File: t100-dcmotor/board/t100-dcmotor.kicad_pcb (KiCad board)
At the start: 2 copper layers, 34.5 x 99.5 mm, 24 parts, among them J1 T100-IN, J2 T100-OUT, J3 Conn_01x08_Female, U1 ATSAMD11D14A-SS, U2 TB67H451FNG, X1 SWD

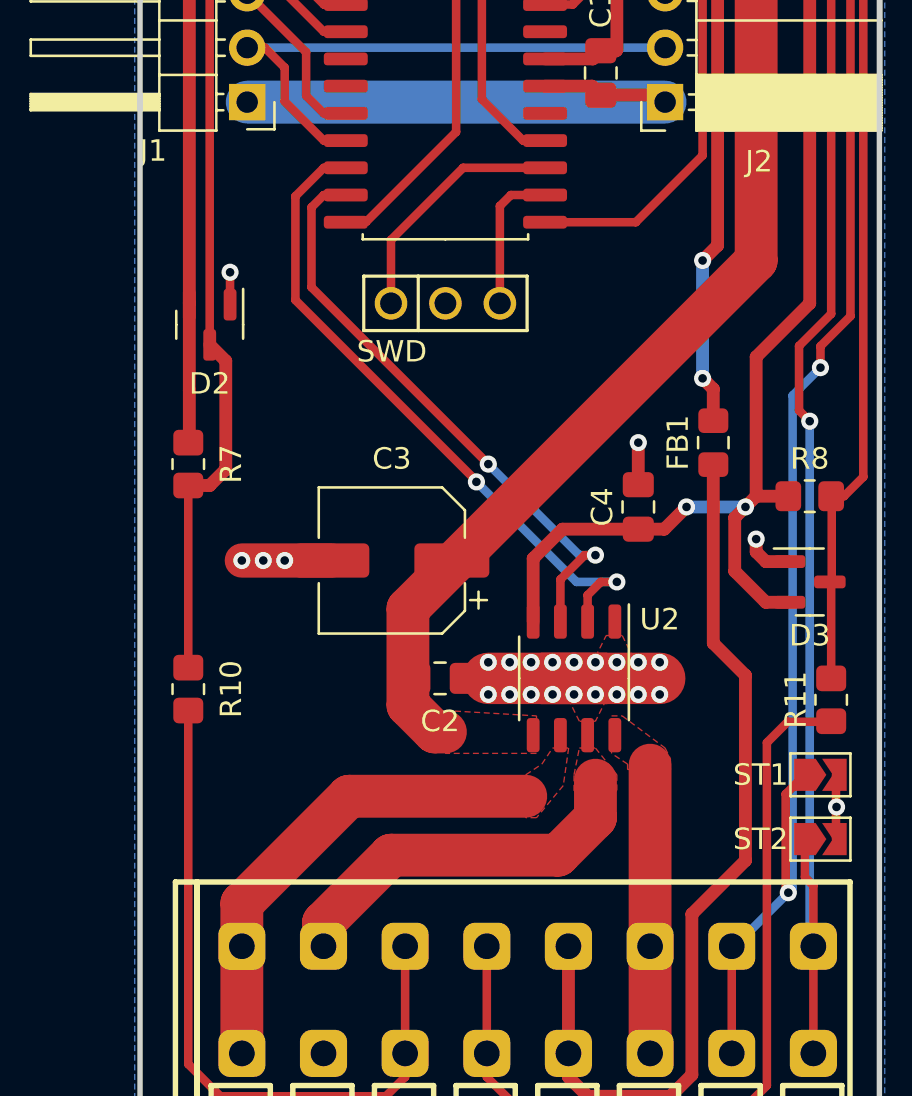
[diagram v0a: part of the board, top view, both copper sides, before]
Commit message: WIP
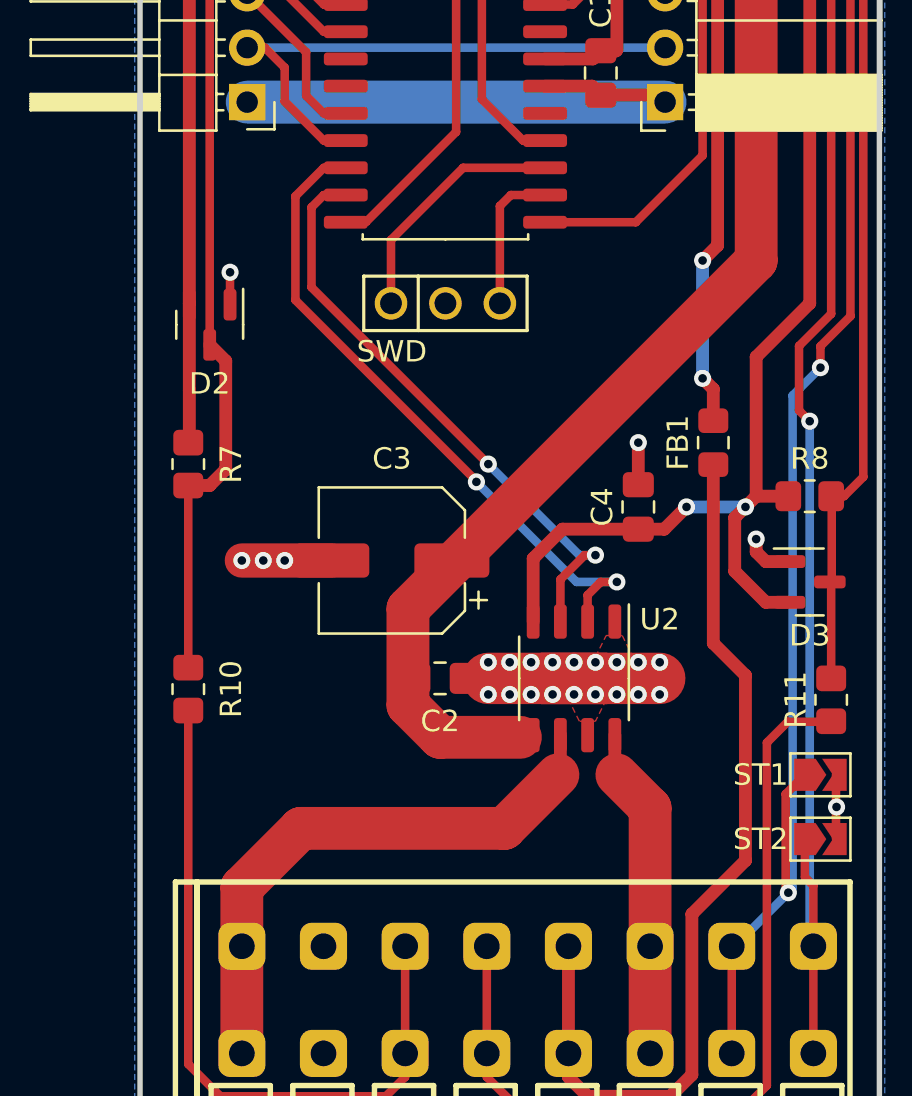
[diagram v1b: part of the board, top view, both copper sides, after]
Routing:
- net GND: track 96.9 -> 79.3 mm
- net /MOTOR_M: track 22.3 -> 26.6 mm
- net +12V: track 102.0 -> 105.6 mm
- net /MOTOR_P: track 13.5 -> 15.5 mm
- removed copper zone on F.Cu, net +12V
- removed copper zone on F.Cu, net /MOTOR_M
- removed copper zone on F.Cu, net /MOTOR_P
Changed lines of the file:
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@@
   )
   (setup
+    (stackup
+      (layer "F.SilkS" (type "Top Silk Screen") (color "White"))
+      (layer "F.Paste" (type "Top Solder Paste"))
+      (layer "F.Mask" (type "Top Solder Mask") (color "Black") (thickness 0.01))
+      (layer "F.Cu" (type "copper") (thickness 0.035))
+      (layer "dielectric 1" (type "core") (thickness 1.51) (material "FR4") (epsilon_r 4.5) (loss_tangent 0.02))
+      (layer "B.Cu" (type "copper") (thickness 0.035))
+      (layer "B.Mask" (type "Bottom Solder Mask") (color "Black") (thickness 0.01))
+      (layer "B.Paste" (type "Bottom Solder Paste"))
+      (layer "B.SilkS" (type "Bottom Silk Screen") (color "White"))
+      (copper_finish "None")
+      (dielectric_constraints no)
+    )
     (pad_to_mask_clearance 0.051)
     (solder_mask_min_width 0.25)
@@
     (property "Sheetname" "")
     (attr through_hole)
-    (fp_text reference "J1" (at 4.385 -2.27 180) (layer "F.SilkS")
+    (fp_text reference "J1" (at 4.385 -2.27 180) (layer "F.SilkS") hide
       (effects (font (size 1 1) (thickness 0.15)))
     )
@@
     (property "Sheetname" "")
     (attr through_hole)
-    (fp_text reference "J2" (at -4.38 -2.77 180) (layer "F.SilkS")
+    (fp_text reference "J2" (at -4.38 -2.77 180) (layer "F.SilkS") hide
       (effects (font (size 1 1) (thickness 0.15)))
     )
@@
   (segment (start 106.915 84.775) (end 107.25 85.11) (width 0.6) (layer "F.Cu") (net 1))
   (segment (start 113 106.55) (end 111.95 106.55) (width 0.6) (layer "F.Cu") (net 1))
-  (segment (start 91.31 124.5) (end 91.31 123.4) (width 2) (layer "F.Cu") (net 1))
   (segment (start 103 112) (end 107 112) (width 2.4) (layer "F.Cu") (net 1))
   (segment (start 115.225 117.975) (end 115.225 119.5) (width 0.4) (layer "F.Cu") (net 1))
-  (segment (start 94.46 120.25) (end 102.25 120.25) (width 2) (layer "F.Cu") (net 1))
   (segment (start 103.84 84.365) (end 104.25 84.775) (width 0.6) (layer "F.Cu") (net 1))
-  (segment (start 104 118.5) (end 104 116.75) (width 2) (layer "F.Cu") (net 1))
   (segment (start 101.65 84.365) (end 103.84 84.365) (width 0.6) (layer "F.Cu") (net 1))
   (segment (start 115.225 116.5) (end 115.225 117.975) (width 0.4) (layer "F.Cu") (net 1))
-  (segment (start 102.25 120.25) (end 104 118.5) (width 2) (layer "F.Cu") (net 1))
   (segment (start 111.95 106.55) (end 111.5 106.1) (width 0.6) (layer "F.Cu") (net 1))
   (segment (start 111.5 106.1) (end 111.5 105.5) (width 0.6) (layer "F.Cu") (net 1))
   (segment (start 106 102.9625) (end 106 101) (width 0.6) (layer "F.Cu") (net 1))
-  (segment (start 91.31 123.4) (end 94.46 120.25) (width 2) (layer "F.Cu") (net 1))
   (segment (start 98.975 71) (end 98.975 64.525) (width 0.4) (layer "F.Cu") (net 1))
   (segment (start 99 112) (end 103 112) (width 2.4) (layer "F.Cu") (net 1))
@@
   (segment (start 87.75 72.41) (end 103.59 72.41) (width 2) (layer "B.Cu") (net 2))
   (segment (start 111 104) (end 108.25 104) (width 0.6) (layer "B.Cu") (net 2))
-  (segment (start 95.25 108.75) (end 95.25 113.25) (width 2) (layer "F.Cu") (net 3))
-  (segment (start 95.25 113.25) (end 96.5 114.5) (width 2) (layer "F.Cu") (net 3))
-  (segment (start 111.5 92.5) (end 95.25 108.75) (width 2) (layer "F.Cu") (net 3))
-  (segment (start 107.25 67.33) (end 109.33 67.33) (width 2) (layer "F.Cu") (net 3))
   (segment (start 111.5 69.5) (end 111.5 92.5) (width 2) (layer "F.Cu") (net 3))
   (segment (start 109.33 67.33) (end 111.5 69.5) (width 2) (layer "F.Cu") (net 3))
-  (segment (start 96.5 114.5) (end 97 114.5) (width 2) (layer "F.Cu") (net 3))
+  (segment (start 107.25 67.33) (end 109.33 67.33) (width 2) (layer "F.Cu") (net 3))
+  (segment (start 111.5 92.5) (end 95.25 108.75) (width 2) (layer "F.Cu") (net 3))
+  (segment (start 95.25 113.25) (end 96.75 114.75) (width 2) (layer "F.Cu") (net 3))
+  (segment (start 95.25 108.75) (end 95.25 113.25) (width 2) (layer "F.Cu") (net 3))
+  (segment (start 96.75 114.75) (end 100.5 114.75) (width 2) (layer "F.Cu") (net 3))
   (segment (start 87.75 64.79) (end 87.75 67.33) (width 2) (layer "B.Cu") (net 3))
   (segment (start 87.75 67.33) (end 107.25 67.33) (width 2) (layer "B.Cu") (net 3))
@@
   (segment (start 91.325 86.905) (end 92.35 86.905) (width 0.4) (layer "F.Cu") (net 11))
   (segment (start 87.75 82.57) (end 107.25 82.57) (width 0.4) (layer "B.Cu") (net 11))
-  (segment (start 106.55 124.5) (end 106.55 116.05) (width 2) (layer "F.Cu") (net 12))
+  (segment (start 104.905 116.405) (end 105 116.5) (width 0.6) (layer "F.Cu") (net 12))
+  (segment (start 106.55 118.05) (end 105 116.5) (width 2) (layer "F.Cu") (net 12))
+  (segment (start 106.55 124.5) (end 106.55 118.05) (width 2) (layer "F.Cu") (net 12))
   (segment (start 106.55 124.5) (end 106.55 129.5) (width 2) (layer "F.Cu") (net 12))
+  (segment (start 104.905 114.65) (end 104.905 116.405) (width 0.6) (layer "F.Cu") (net 12))
   (segment (start 115 114.025) (end 112.975 114.025) (width 0.4) (layer "F.Cu") (net 13))
   (segment (start 112.975 114.025) (end 112 115) (width 0.4) (layer "F.Cu") (net 13))
@@
   (segment (start 85 113.5) (end 85 130) (width 0.4) (layer "F.Cu") (net 14))
   (segment (start 95.12 130.6) (end 95.12 129.5) (width 0.4) (layer "F.Cu") (net 14))
-  (segment (start 87.5 124.5) (end 87.5 122.5) (width 2) (layer "F.Cu") (net 15))
-  (segment (start 92.5 117.5) (end 100.75 117.5) (width 2) (layer "F.Cu") (net 15))
+  (segment (start 87.5 124.5) (end 87.5 121.75) (width 2) (layer "F.Cu") (net 15))
+  (segment (start 99.75 119) (end 102.25 116.5) (width 2) (layer "F.Cu") (net 15))
   (segment (start 87.5 124.5) (end 87.5 129.5) (width 2) (layer "F.Cu") (net 15))
-  (segment (start 87.5 122.5) (end 92.5 117.5) (width 2) (layer "F.Cu") (net 15))
+  (segment (start 87.5 121.75) (end 90.25 119) (width 2) (layer "F.Cu") (net 15))
+  (segment (start 102.365 116.385) (end 102.25 116.5) (width 0.6) (layer "F.Cu") (net 15))
+  (segment (start 102.365 114.65) (end 102.365 116.385) (width 0.6) (layer "F.Cu") (net 15))
+  (segment (start 90.25 119) (end 99.75 119) (width 2) (layer "F.Cu") (net 15))
   (segment (start 98.699999 84.979999) (end 100.625 86.905) (width 0.4) (layer "F.Cu") (net 16))
   (segment (start 99 75.2) (end 98.699999 75.500001) (width 0.4) (layer "F.Cu") (net 16))
@@
   (segment (start 109 76.7) (end 109 87.599241) (width 0.4) (layer "F.Cu") (net 24))
   (segment (start 87.75 74.95) (end 107.25 74.95) (width 0.4) (layer "B.Cu") (net 24))
-  (zone (net 12) (net_name "/MOTOR_P") (layer "F.Cu") (name "GND") (hatch edge 0.508)
-    (connect_pads yes (clearance 0))
-    (min_thickness 0.254) (filled_areas_thickness no)
-    (fill yes (thermal_gap 0.508) (thermal_bridge_width 0.508))
-    (polygon
-      (pts
-        (xy 107.25 115.25)
-        (xy 107.5 115.75)
-        (xy 107.5 116.25)
-        (xy 105.5 116.25)
-        (xy 105.5 116)
-        (xy 104.75 115.5)
-        (xy 104.75 113.75)
-        (xy 105.25 113.75)
-      )
-    )
-  )
   (zone (net 1) (net_name "GND") (layer "F.Cu") (name "GND") (hatch edge 0.508)
     (connect_pads yes (clearance 0))
@@
       )
     )
-  )
-  (zone (net 3) (net_name "+12V") (layer "F.Cu") (name "GND") (hatch edge 0.508)
-    (connect_pads yes (clearance 0))
-    (min_thickness 0.254) (filled_areas_thickness no)
-    (fill yes (thermal_gap 0.508) (thermal_bridge_width 0.508))
-    (polygon
-      (pts
-        (xy 101.25 115.5)
-        (xy 97 115.5)
-        (xy 97 113.5)
-        (xy 101.25 113.75)
-      )
-    )
-  )
-  (zone (net 15) (net_name "/MOTOR_M") (layer "F.Cu") (name "GND") (hatch full 0.508)
-    (connect_pads yes (clearance 0))
-    (min_thickness 0.254) (filled_areas_thickness no)
-    (fill yes (thermal_gap 0.508) (thermal_bridge_width 0.508))
-    (polygon
-      (pts
-        (xy 102.5 117)
-        (xy 101.25 118.5)
-        (xy 100.75 118.5)
-        (xy 100.75 116.5)
-        (xy 101.5 116)
-        (xy 102 115.25)
-        (xy 102.75 115.25)
-      )
-    )
-  )
-  (zone (net 1) (net_name "GND") (layer "F.Cu") (name "GND") (hatch edge 0.508)
-    (connect_pads yes (clearance 0))
-    (min_thickness 0.254) (filled_areas_thickness no)
-    (fill yes (thermal_gap 0.508) (thermal_bridge_width 0.508))
-    (polygon
-      (pts
-        (xy 105 116.5)
-        (xy 105 117.25)
-        (xy 103 117.25)
-        (xy 103 116.5)
-        (xy 103.25 115.25)
-        (xy 104 115.25)
-      )
-    )

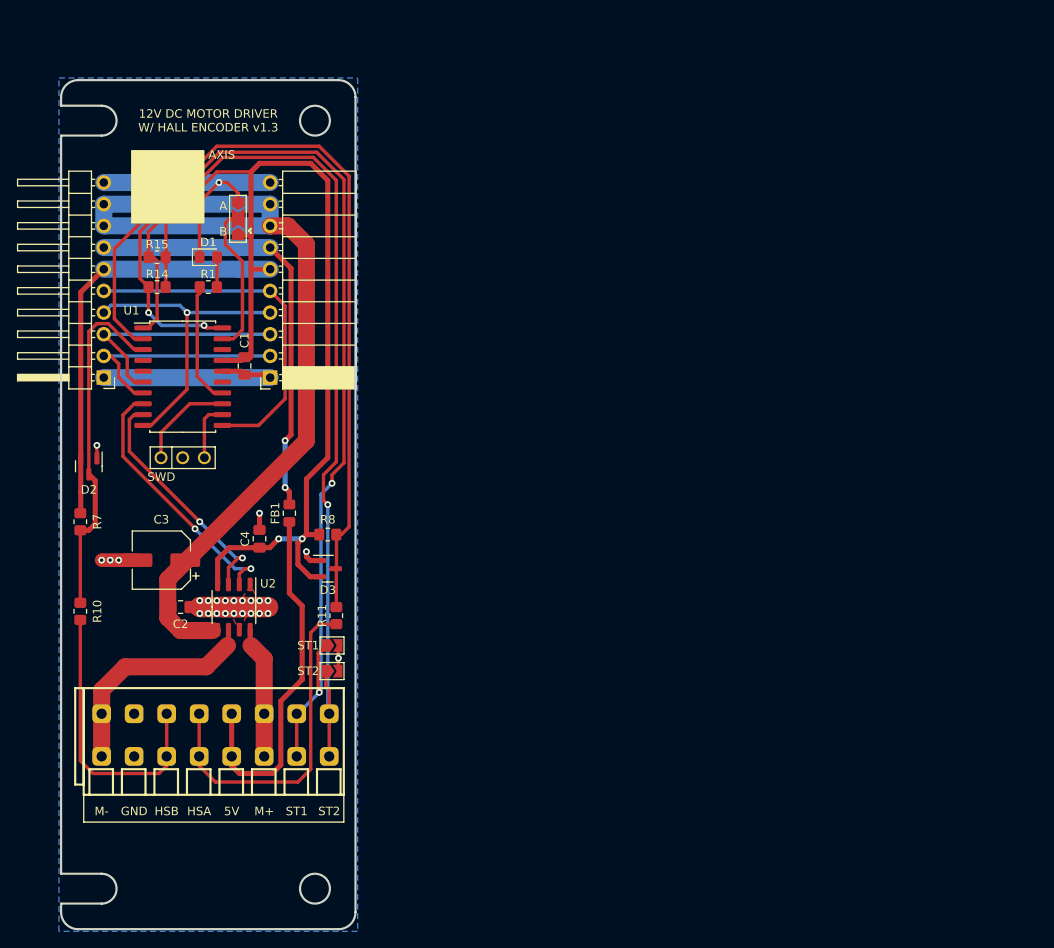
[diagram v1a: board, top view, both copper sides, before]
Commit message: WIP
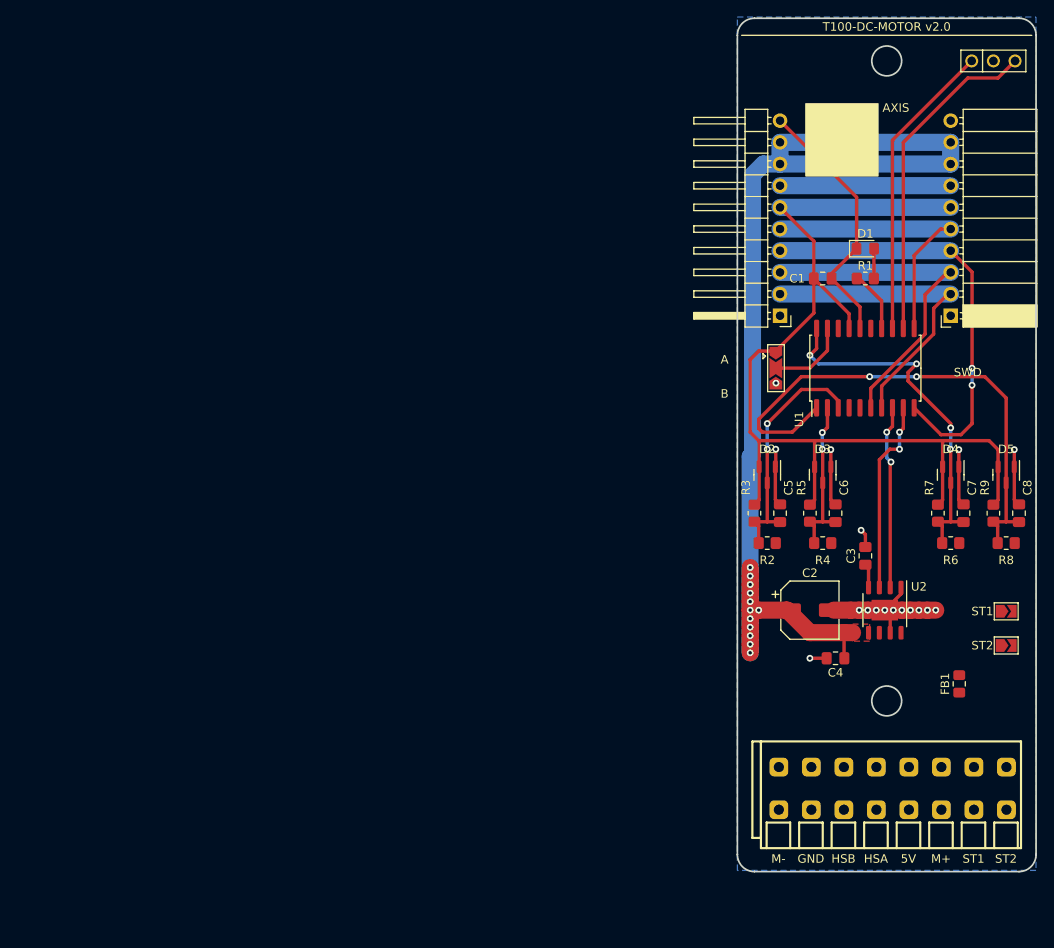
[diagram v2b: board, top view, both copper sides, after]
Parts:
- removed R10, R11: 270R, Resistor_SMD:R_0805_2012Metric_Pad1.20x1.40mm_HandSolder
- removed R14, R15: 10k, Resistor_SMD:R_0805_2012Metric_Pad1.20x1.40mm_HandSolder
- added C5: C, Capacitor_SMD:C_0805_2012Metric_Pad1.18x1.45mm_HandSolder, F.Cu at (167.0, 101.0)
- added C6: C, Capacitor_SMD:C_0805_2012Metric_Pad1.18x1.45mm_HandSolder, F.Cu at (173.5, 101.0)
- added C7: C, Capacitor_SMD:C_0805_2012Metric_Pad1.18x1.45mm_HandSolder, F.Cu at (188.5, 101.0)
- added C8: C, Capacitor_SMD:C_0805_2012Metric_Pad1.18x1.45mm_HandSolder, F.Cu at (195.0, 101.0)
- added D4: BAT54S, Package_TO_SOT_SMD:SOT-23, F.Cu at (187.0, 96.5)
- added D5: BAT54S, Package_TO_SOT_SMD:SOT-23, F.Cu at (193.5, 96.5)
- added R2: R, Resistor_SMD:R_0805_2012Metric_Pad1.20x1.40mm_HandSolder, F.Cu at (165.5, 104.5)
- added R3: R, Resistor_SMD:R_0805_2012Metric_Pad1.20x1.40mm_HandSolder, F.Cu at (164.0, 101.0)
- added R4: R, Resistor_SMD:R_0805_2012Metric_Pad1.20x1.40mm_HandSolder, F.Cu at (172.0, 104.5)
- added R5: R, Resistor_SMD:R_0805_2012Metric_Pad1.20x1.40mm_HandSolder, F.Cu at (170.5, 101.0)
- added R6: R, Resistor_SMD:R_0805_2012Metric_Pad1.20x1.40mm_HandSolder, F.Cu at (187.0, 104.5)
- added R9: R, Resistor_SMD:R_0805_2012Metric_Pad1.20x1.40mm_HandSolder, F.Cu at (192.0, 101.0)
- C2: value 100n -> 100u/16V; footprint Capacitor_SMD:C_0805_2012Metric_Pad1.18x1.45mm_HandSolder -> Capacitor_SMD:CP_Elec_6.3x5.4
- C3: value 100u/16V -> 100n; footprint Capacitor_SMD:CP_Elec_6.3x5.4 -> Capacitor_SMD:C_0805_2012Metric_Pad1.18x1.45mm_HandSolder
- R7, R8: value 10k -> R
- moved X1 105.8 mm to (192.0, 48.0)
- moved R7 100.5 mm to (185.5, 101.0), turned to -90 degrees
- moved C3 82.5 mm to (177.0, 106.0), turned to 90 degrees
- moved FB1 81.0 mm to (188.0, 121.0)
- moved J2 80.1 mm to (187.0, 77.9)
- moved U1 80.0 mm to (177.0, 84.0), turned to 90 degrees
- moved J3 79.6 mm to (166.9, 130.8)
- moved J1 79.6 mm to (167.0, 77.9)
- moved D2 79.5 mm to (165.5, 96.5)
- moved R8 79.5 mm to (193.5, 104.5), turned to 0 degrees
- moved ST1 79.1 mm to (193.5, 112.5)
- moved ST2 79.1 mm to (193.5, 116.5)
- moved D1 77.0 mm to (177.0, 70.0)
- moved R1 77.0 mm to (177.0, 73.5)
- moved U2 76.3 mm to (179.3, 112.4)
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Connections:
- C3 pad 1: +12V -> +3V3
- C4 pad 1: +3V3 -> +12V
- J3 pad 3: Net-(J3-Pad3) -> /input-filter/PORT
- J3 pad 4: Net-(J3-Pad4) -> /input-filter1/PORT
- J3 pad 7: /STOP_1 -> /input-filter2/PORT
- J3 pad 8: /STOP_2 -> /input-filter3/PORT
- R7 pad 1: /HALL_B -> +3V3
- R7 pad 2: +3V3 -> /STOP_1
- R8 pad 1: /HALL_A -> /STOP_2
- R8 pad 2: +3V3 -> /input-filter3/PORT
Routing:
- net /STOP_1: track 124.3 -> 43.1 mm
- net /HALL_A: track 97.9 -> 19.4 mm, vias 0 -> 2
- net /STOP_2: track 113.4 -> 61.5 mm, vias 1 -> 2
- net +3V3: track 173.3 -> 122.5 mm, vias 2 -> 0
- net Net-(FB1-Pad1): track 42.8 -> 0.00 mm
- net Net-(J3-Pad4): track 40.0 -> 0.00 mm
- net Net-(J3-Pad3): track 33.7 -> 0.00 mm
- net /SWCLK: track 6.86 -> 38.8 mm
- net +5V: track 51.1 -> 20.0 mm, vias 2 -> 0
- net /MOTOR_M: track 26.6 -> 0.00 mm
- net +12V: track 105.6 -> 131.1 mm, vias 0 -> 12
- net /SWDIO: track 11.5 -> 35.2 mm
- net /MOTOR_P: track 15.5 -> 0.00 mm
- net /IRQ: track 36.1 -> 49.9 mm, vias 1 -> 2
- net /HALL_B: track 41.4 -> 28.6 mm, vias 0 -> 2
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- added copper zone on F.Cu, net +12V
- removed copper zone on F.Cu, net GND
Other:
- board size 34.5 x 99.5 mm -> 35 x 100 mm
- board text added: "T100-DC-MOTOR v2.0"
- board text removed: "12V DC MOTOR DRIVER W/ HALL ENCODER v1.3"
